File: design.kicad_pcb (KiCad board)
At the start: 2 copper layers, 50 x 30 mm, 20 parts, among them J1 Conn_02x02_Counter_Clockwise, J2 Conn_02x02_Counter_Clockwise, J3 Conn_02x02_Counter_Clockwise, J4 Conn_02x02_Counter_Clockwise, U1 TPS63900

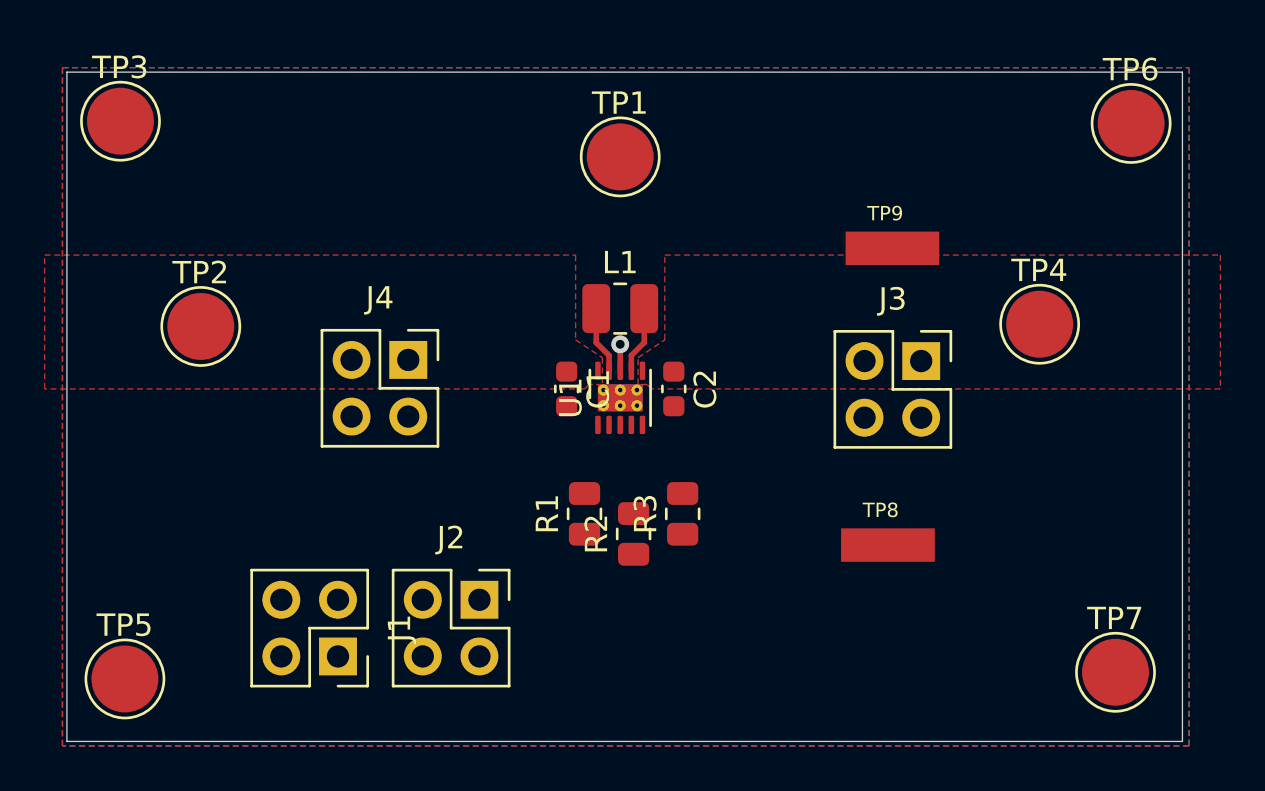
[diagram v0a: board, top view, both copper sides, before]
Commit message: update
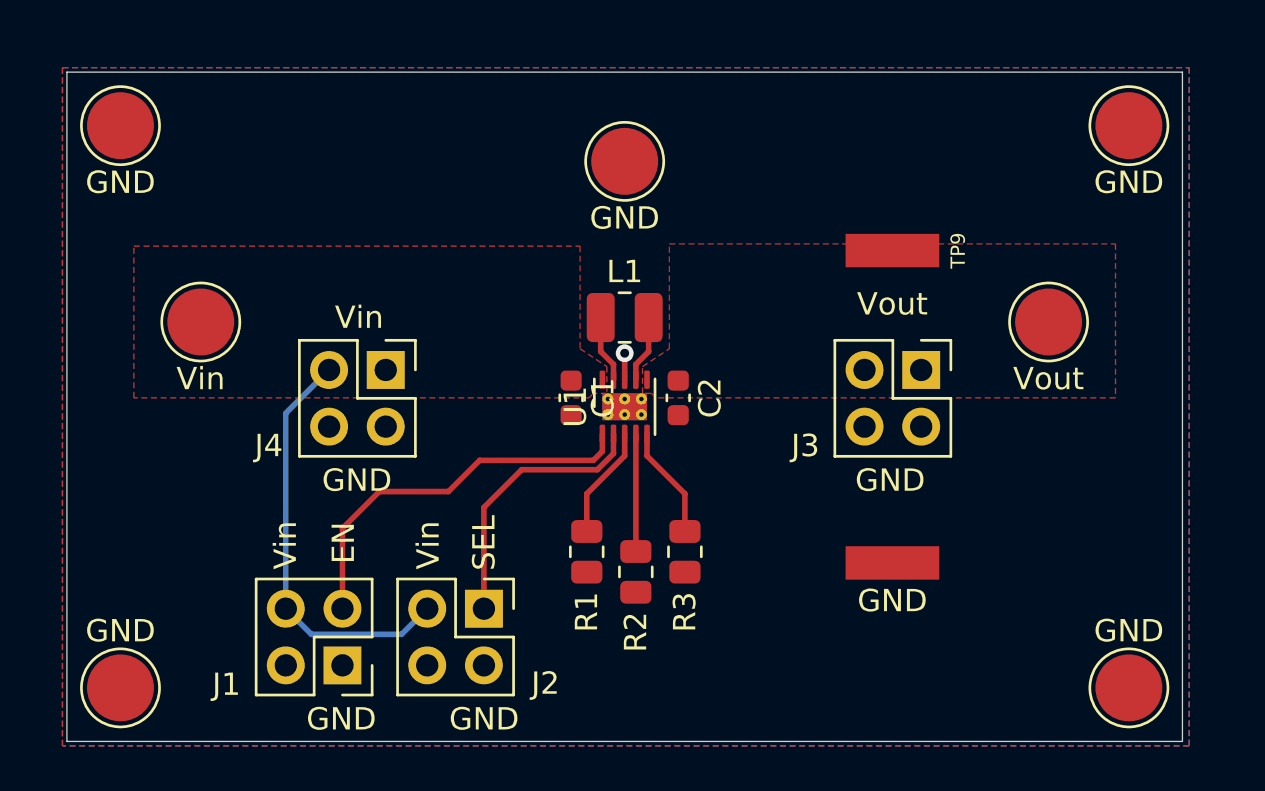
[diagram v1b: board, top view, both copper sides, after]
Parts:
- TP1, TP3, TP5, TP6, TP7: value TestPoint -> GND
- TP2: value TestPoint -> Vin
- TP4: value TestPoint -> Vout
- moved R1 1.70 mm to (164.7, 111.9)
- moved R2 1.70 mm to (166.9, 112.8)
- moved R3 1.70 mm to (169.1, 111.9)
- moved J4 1.11 mm to (155.7, 103.8)
- moved TP7 0.92 mm to (189.0, 118.0), turned to 180 degrees
- moved TP8 0.82 mm to (178.4, 112.4)
- moved C2 0.45 mm to (168.8, 105.0)
- moved J2 0.45 mm to (160.1, 114.5)
- moved L1 0.45 mm to (166.4, 101.4)
- moved U1 0.45 mm to (166.4, 105.4)
- moved C1 0.45 mm to (164.0, 105.0)
- moved TP5 0.45 mm to (143.8, 118.0), turned to 180 degrees
- moved J1 0.45 mm to (153.8, 117.0)
- moved TP4 0.41 mm to (185.4, 101.6)
- moved J3 0.40 mm to (179.7, 103.8)
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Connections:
- J1 pad 1: unconnected-(J1-Pad1) -> GND
- J1 pad 3: GND -> unconnected-(J1-Pad3)
- R1 pad 1: Net-(R1-Pad1) -> GND
- R3 pad 1: Net-(R1-Pad1) -> GND
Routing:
- net Vin: track 0.00 -> 18.8 mm
- net EN: track 0.00 -> 17.5 mm
- net SEL: track 0.00 -> 12.2 mm
- net Net-(R2-Pad2): track 0.00 -> 5.28 mm
- net Net-(R1-Pad2): track 0.00 -> 5.08 mm
- net Net-(R3-Pad2): track 0.00 -> 5.08 mm
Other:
- board text added: "EN"
- board text added: "GND"
- board text added: "SEL"
- board text added: "Vin"
- board text added: "Vout"
